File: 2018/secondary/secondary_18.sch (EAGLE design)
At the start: 35 parts, among them Q1 BUZ11BV, Q2 BUZ11BV

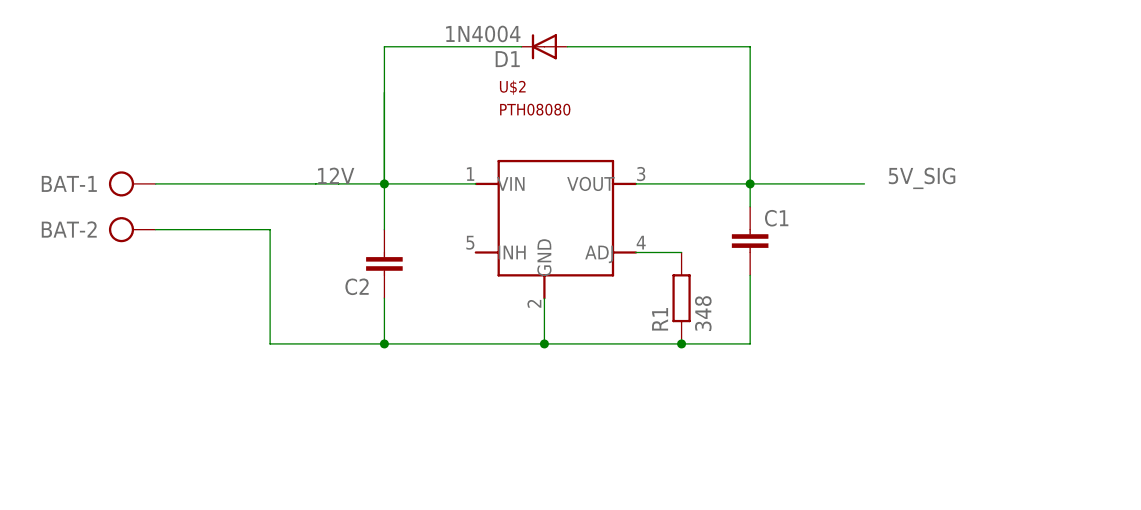
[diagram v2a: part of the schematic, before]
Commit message: [secondary] Adds the final board
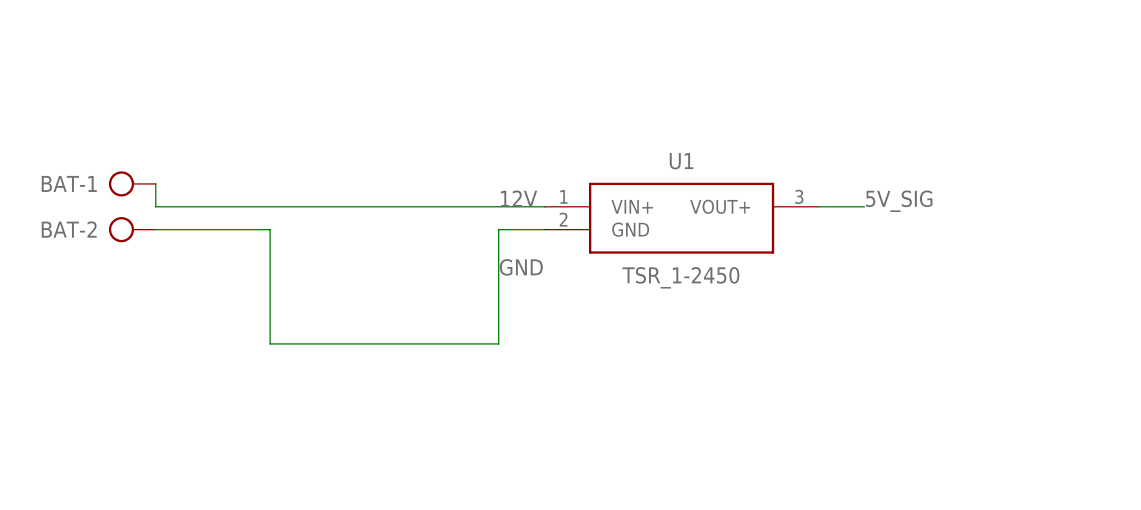
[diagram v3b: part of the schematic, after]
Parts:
- removed C1, C2: (no value), rcl:C-EU025-060X050
- removed D1: 1N4004, diode:1N4004
- removed R1: 348, resistor:R-EU_0204/7
- removed U$2: PTH08080, pth08080:PTH08080
- added U1: TSR_1-2450, SamacSys_Parts:TSR_1-2450
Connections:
- removed net N$1: R1.2, U$2.ADJ
- net 12V: now also U1.VIN+; no longer C2.2, D1.C, U$2.VIN
- net 5V_SIG: now also U1.VOUT+; no longer C1.1, D1.A, U$2.VOUT
- net GND: now also U1.GND; no longer C1.2, C2.1, R1.1, U$2.GND
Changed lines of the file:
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@@
 <?xml version="1.0" encoding="utf-8"?>
 <!DOCTYPE eagle SYSTEM "eagle.dtd">
-<eagle version="6.1">
+<eagle version="8.6.0">
 <drawing>
 <settings>
 <setting alwaysvectorfont="no"/>
+<setting keepoldvectorfont="yes"/>
 <setting verticaltext="up"/>
 </settings>
@@
 <parts>
 <part name="U$1" library="Teensy356" deviceset="TEENSY_3.5/3.6" device=""/>
-<part name="U$2" library="pth08080" deviceset="PTH08080" device=""/>
-<part name="R1" library="resistor" deviceset="R-EU_" device="0204/7" value="348"/>
-<part name="C1" library="rcl" deviceset="C-EU" device="025-060X050"/>
-<part name="C2" library="rcl" deviceset="C-EU" device="025-060X050"/>
-<part name="D1" library="diode" deviceset="1N4004" device=""/>
 <part name="BAT" library="con-ptr500" deviceset="AK300/2" device=""/>
 <part name="CON_MOT1" library="con-lstb" deviceset="MA03-1" device=""/>
@@
 <part name="JP1" library="pinhead" deviceset="PINHD-1X2" device=""/>
 <part name="JP2" library="pinhead" deviceset="PINHD-1X2" device=""/>
+<part name="U1" library="SamacSys_Parts" deviceset="TSR_1-2450" device=""/>
 </parts>
 <sheets>
@@
 <instances>
 <instance part="U$1" gate="G$1" x="83.82" y="60.96"/>
-<instance part="U$2" gate="G$1" x="-38.1" y="137.16"/>
-<instance part="R1" gate="G$1" x="-25.4" y="127" rot="R90"/>
-<instance part="C1" gate="G$1" x="-17.78" y="134.62"/>
-<instance part="C2" gate="G$1" x="-58.42" y="129.54" rot="R180"/>
-<instance part="D1" gate="1" x="-40.64" y="154.94" rot="R180"/>
 <instance part="BAT" gate="-1" x="-88.9" y="139.7"/>
 <instance part="BAT" gate="-2" x="-88.9" y="134.62"/>
@@
 <instance part="JP1" gate="G$1" x="185.42" y="15.24"/>
 <instance part="JP2" gate="G$1" x="180.34" y="-12.7"/>
+<instance part="U1" gate="G$1" x="-40.64" y="137.16"/>
 </instances>
 <busses>
 </busses>
 <nets>
-<net name="N$1" class="0">
-<segment>
-<pinref part="U$2" gate="G$1" pin="ADJ"/>
-<pinref part="R1" gate="G$1" pin="2"/>
-<wire x1="-30.48" y1="132.08" x2="-25.4" y2="132.08" width="0.1524" layer="91"/>
-</segment>
-</net>
 <net name="GND" class="0">
 <segment>
-<pinref part="R1" gate="G$1" pin="1"/>
-<pinref part="U$2" gate="G$1" pin="GND"/>
-<wire x1="-25.4" y1="121.92" x2="-40.64" y2="121.92" width="0.1524" layer="91"/>
-<wire x1="-40.64" y1="127" x2="-40.64" y2="121.92" width="0.1524" layer="91"/>
-<pinref part="C1" gate="G$1" pin="2"/>
-<wire x1="-17.78" y1="129.54" x2="-17.78" y2="121.92" width="0.1524" layer="91"/>
-<wire x1="-17.78" y1="121.92" x2="-25.4" y2="121.92" width="0.1524" layer="91"/>
-<junction x="-25.4" y="121.92"/>
-<pinref part="C2" gate="G$1" pin="1"/>
-<wire x1="-58.42" y1="127" x2="-58.42" y2="121.92" width="0.1524" layer="91"/>
-<wire x1="-58.42" y1="121.92" x2="-40.64" y2="121.92" width="0.1524" layer="91"/>
-<junction x="-40.64" y="121.92"/>
 <pinref part="BAT" gate="-2" pin="KL"/>
 <wire x1="-83.82" y1="134.62" x2="-71.12" y2="134.62" width="0.1524" layer="91"/>
 <wire x1="-71.12" y1="134.62" x2="-71.12" y2="121.92" width="0.1524" layer="91"/>
-<wire x1="-71.12" y1="121.92" x2="-58.42" y2="121.92" width="0.1524" layer="91"/>
-<junction x="-58.42" y="121.92"/>
+<pinref part="U1" gate="G$1" pin="GND"/>
+<wire x1="-40.64" y1="134.62" x2="-45.72" y2="134.62" width="0.1524" layer="91"/>
+<wire x1="-71.12" y1="121.92" x2="-45.72" y2="121.92" width="0.1524" layer="91"/>
+<wire x1="-45.72" y1="121.92" x2="-45.72" y2="134.62" width="0.1524" layer="91"/>
+<label x="-45.72" y="129.54" size="1.778" layer="95"/>
 </segment>
 <segment>
@@
 <net name="12V" class="0">
 <segment>
-<pinref part="U$2" gate="G$1" pin="VIN"/>
-<pinref part="C2" gate="G$1" pin="2"/>
-<wire x1="-48.26" y1="139.7" x2="-58.42" y2="139.7" width="0.1524" layer="91"/>
-<wire x1="-58.42" y1="139.7" x2="-58.42" y2="134.62" width="0.1524" layer="91"/>
-<wire x1="-58.42" y1="139.7" x2="-58.42" y2="149.86" width="0.1524" layer="91"/>
-<junction x="-58.42" y="139.7"/>
-<label x="-66.04" y="139.7" size="1.778" layer="95"/>
-<pinref part="D1" gate="1" pin="C"/>
-<wire x1="-43.18" y1="154.94" x2="-58.42" y2="154.94" width="0.1524" layer="91"/>
-<wire x1="-58.42" y1="154.94" x2="-58.42" y2="139.7" width="0.1524" layer="91"/>
-<wire x1="-58.42" y1="139.7" x2="-63.5" y2="139.7" width="0.1524" layer="91"/>
-<pinref part="BAT" gate="-1" pin="KL"/>
-<wire x1="-63.5" y1="139.7" x2="-66.04" y2="139.7" width="0.1524" layer="91"/>
-<wire x1="-83.82" y1="139.7" x2="-66.04" y2="139.7" width="0.1524" layer="91"/>
-</segment>
-<segment>
 <label x="154.94" y="-5.08" size="1.778" layer="95"/>
 <pinref part="D2" gate="1" pin="C"/>
@@
 <label x="53.34" y="139.7" size="1.778" layer="95"/>
 </segment>
+<segment>
+<pinref part="U1" gate="G$1" pin="VIN+"/>
+<label x="-45.72" y="137.16" size="1.778" layer="95"/>
+<pinref part="BAT" gate="-1" pin="KL"/>
+<wire x1="-40.64" y1="137.16" x2="-83.82" y2="137.16" width="0.1524" layer="91"/>
+<wire x1="-83.82" y1="137.16" x2="-83.82" y2="139.7" width="0.1524" layer="91"/>
+</segment>
 </net>
 <net name="5V_SIG" class="0">
-<segment>
-<pinref part="U$2" gate="G$1" pin="VOUT"/>
-<pinref part="C1" gate="G$1" pin="1"/>
-<wire x1="-30.48" y1="139.7" x2="-17.78" y2="139.7" width="0.1524" layer="91"/>
-<wire x1="-17.78" y1="139.7" x2="-17.78" y2="137.16" width="0.1524" layer="91"/>
-<wire x1="-17.78" y1="139.7" x2="-5.08" y2="139.7" width="0.1524" layer="91"/>
-<junction x="-17.78" y="139.7"/>
-<label x="-2.54" y="139.7" size="1.778" layer="95"/>
-<pinref part="D1" gate="1" pin="A"/>
-<wire x1="-17.78" y1="139.7" x2="-17.78" y2="154.94" width="0.1524" layer="91"/>
-<wire x1="-17.78" y1="154.94" x2="-38.1" y2="154.94" width="0.1524" layer="91"/>
-</segment>
 <segment>
 <pinref part="U$1" gate="G$1" pin="VIN"/>
@@
 <wire x1="-2.54" y1="50.8" x2="0" y2="50.8" width="0.1524" layer="91"/>
 <label x="0" y="50.8" size="1.778" layer="95"/>
+</segment>
+<segment>
+<pinref part="U1" gate="G$1" pin="VOUT+"/>
+<wire x1="-10.16" y1="137.16" x2="-5.08" y2="137.16" width="0.1524" layer="91"/>
+<label x="-5.08" y="137.16" size="1.778" layer="95"/>
 </segment>
 </net>
@@
 </schematic>
 </drawing>
+<compatibility>
+<note version="6.3" minversion="6.2.2" severity="warning">
+Since Version 6.2.2 text objects can contain more than one line,
+which will not be processed correctly with this version.
+</note>
+</compatibility>
 </eagle>
